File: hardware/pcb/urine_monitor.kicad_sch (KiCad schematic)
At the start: 27 parts, among them J1 LoadCell, J2 EInk_FPC, J3 USB-C_Power, J4 I2C+BOOT0+PWR, Q1 SI2301, Q2 2N7002, SW1 USER_BTN, U1 RAK3172, U2 HX711, U3 TPS61220, U4 MIC5504-3.3

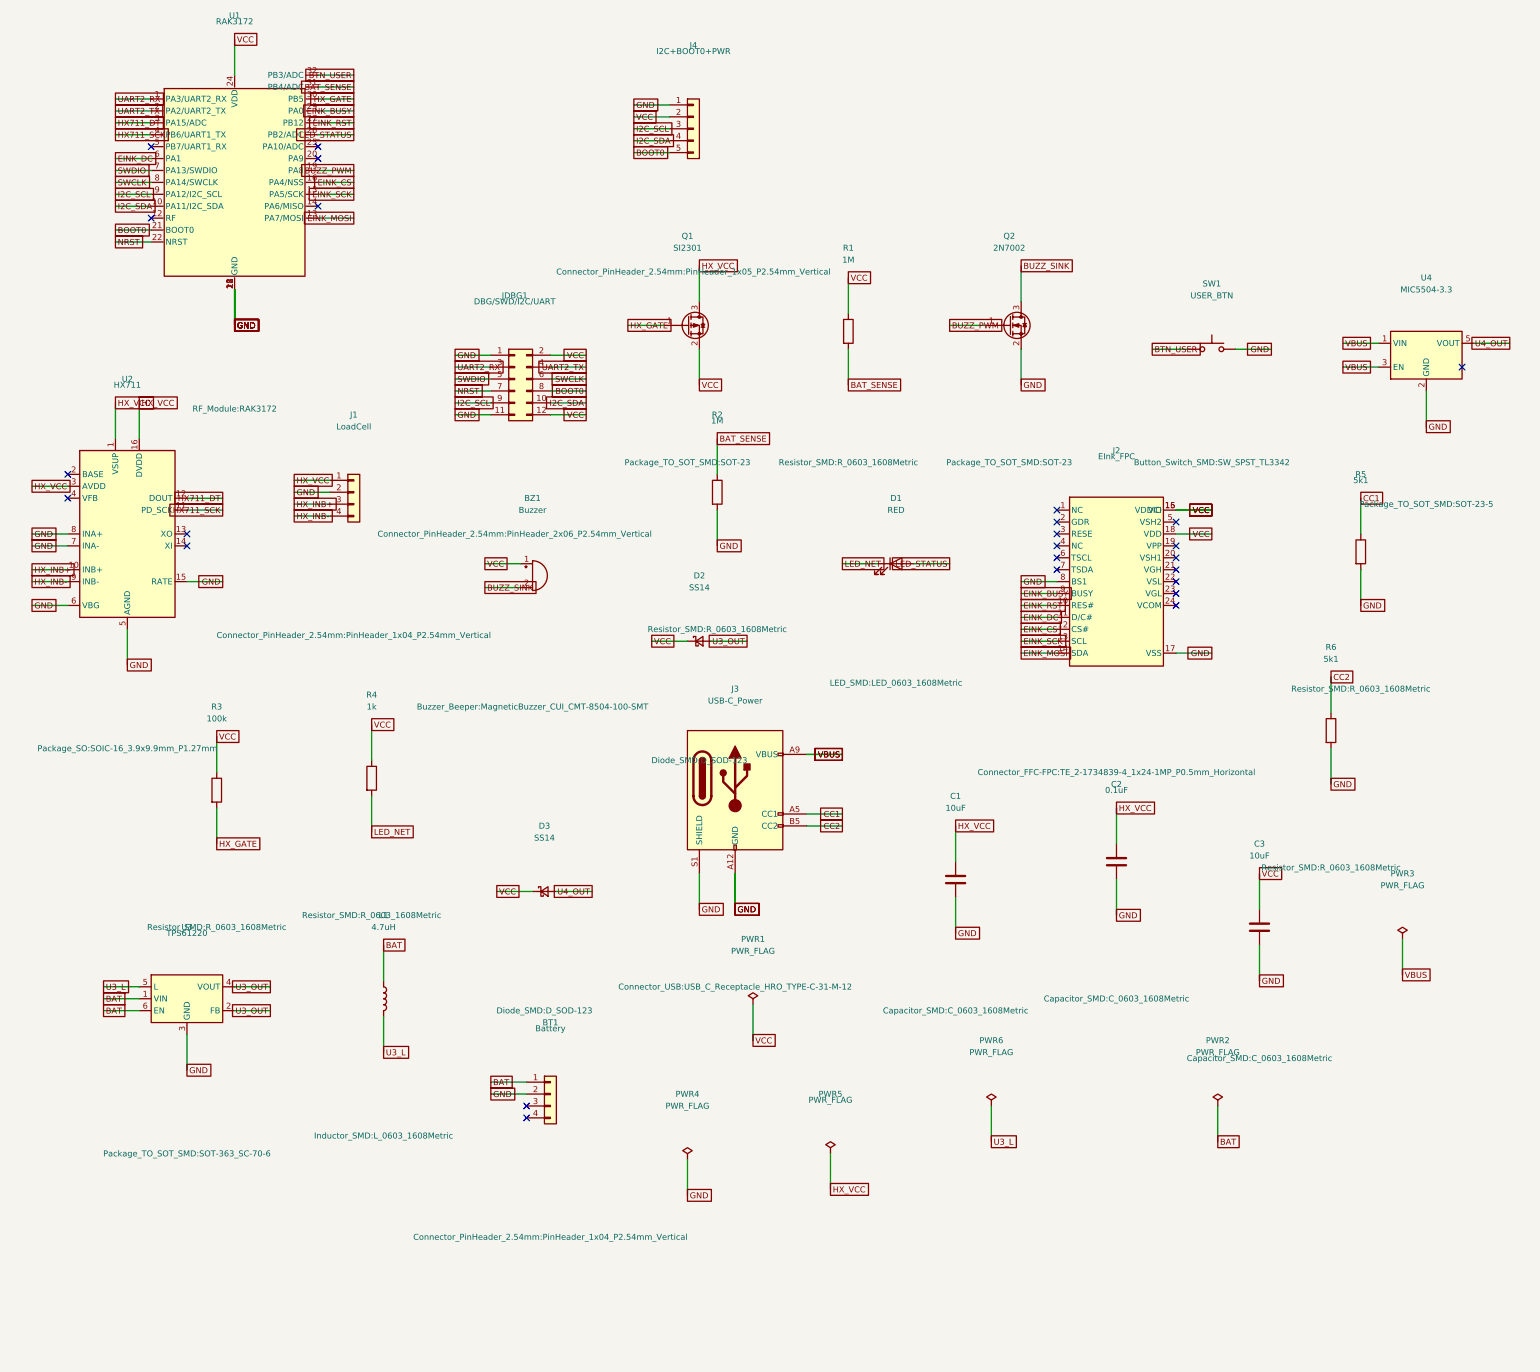
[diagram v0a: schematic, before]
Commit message: init
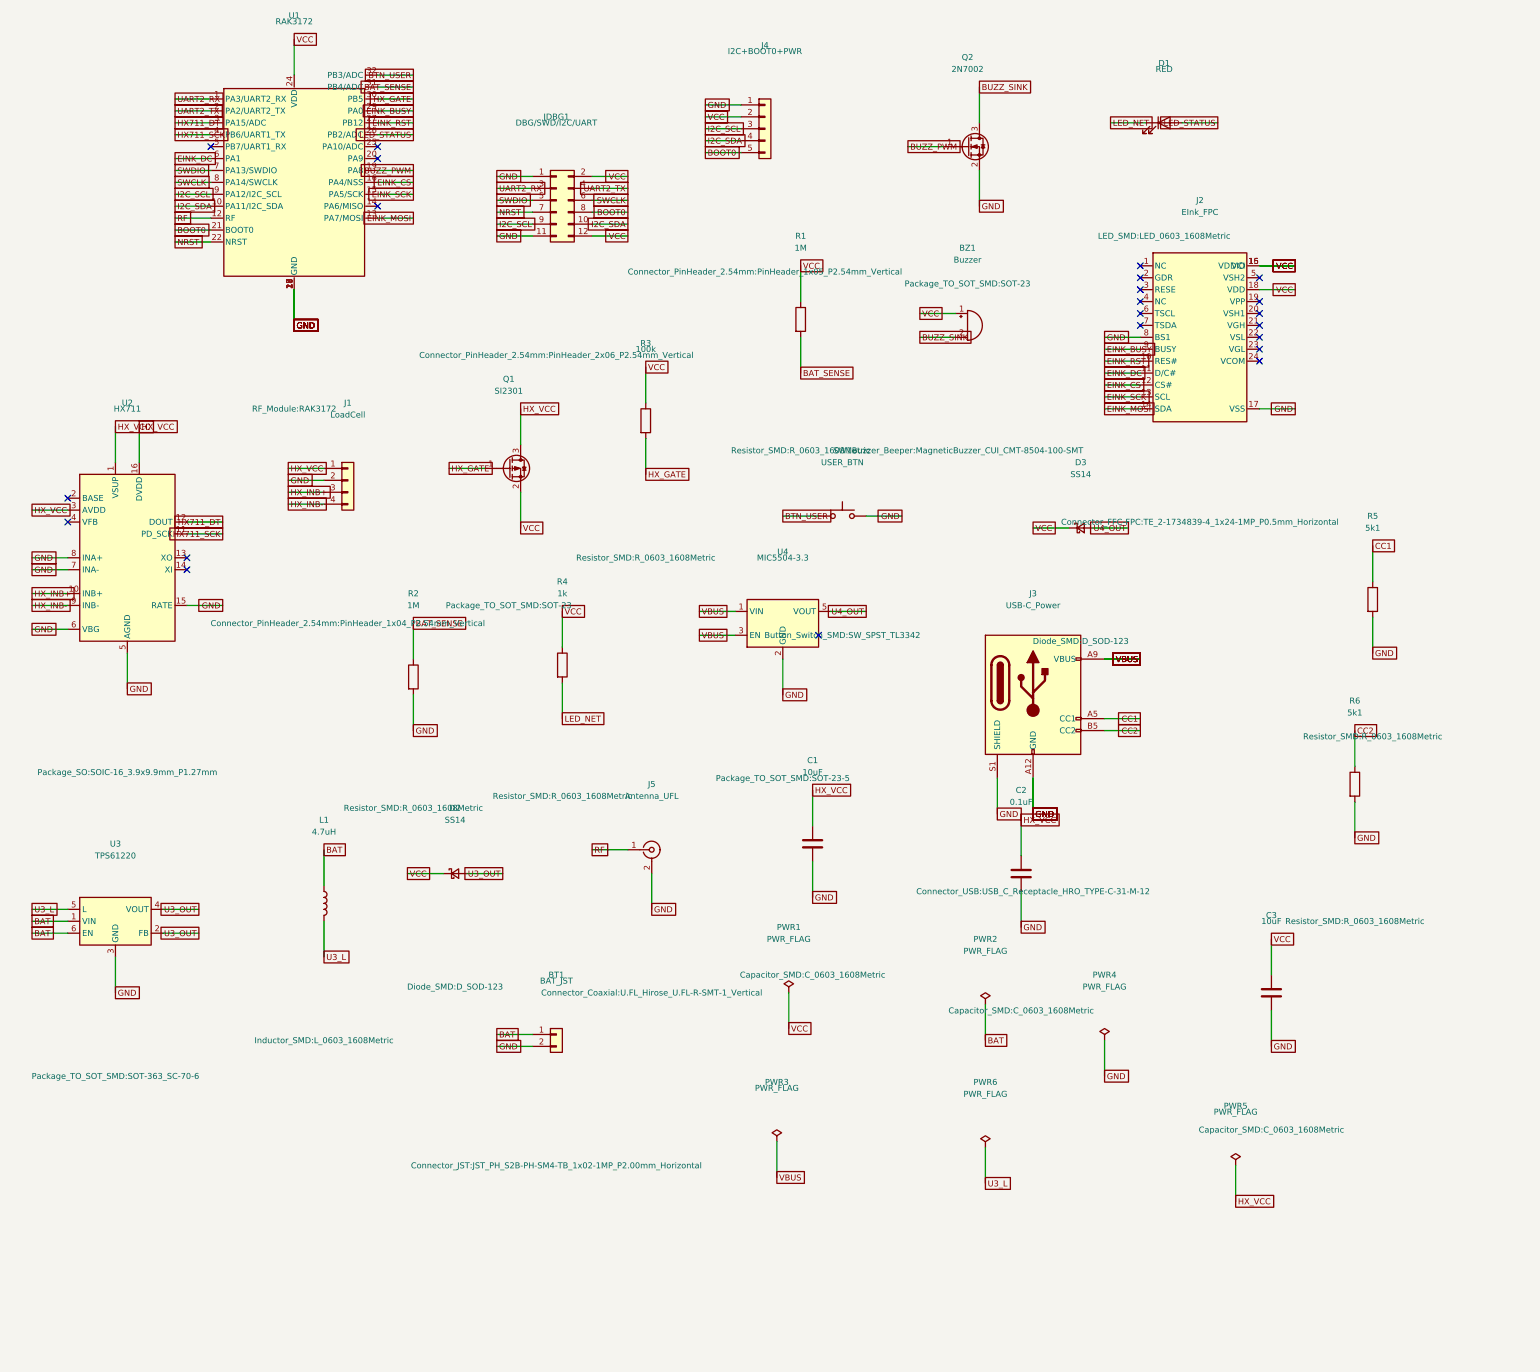
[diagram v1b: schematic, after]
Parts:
- removed BT1: Battery, Connector_PinHeader_2.54mm:PinHeader_1x04_P2.54mm_Vertical, symbol Connector_Generic:Conn_01x04
- removed J3: USB-C_Power, Connector_USB:USB_C_Receptacle_HRO_TYPE-C-31-M-12, symbol Connector:USB_C_Receptacle_PowerOnly_6P
- added BT1: BAT_JST, Connector_JST:JST_PH_S2B-PH-SM4-TB_1x02-1MP_P2.00mm_Horizontal, symbol Connector_Generic:Conn_01x02
- added J3: USB-C_Power, Connector_USB:USB_C_Receptacle_HRO_TYPE-C-31-M-12, symbol Connector:USB_C_Receptacle_PowerOnly_24P
- added J5: Antenna_UFL, Connector_Coaxial:U.FL_Hirose_U.FL-R-SMT-1_Vertical, symbol Connector:Conn_Coaxial
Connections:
- net BAT: now also BT1.1 (Pin_1)
- net CC1: now also J3.A5 (CC1)
- net CC2: now also J3.B5 (CC2)
- net GND: now also BT1.2 (Pin_2), J3.A1 (GND), J3.A12 (GND), J3.B1 (GND), J3.B12 (GND), J3.S1 (SHIELD), J5.2 (Ext)
- net VBUS: now also J3.A4 (VBUS), J3.A9 (VBUS), J3.B4 (VBUS), J3.B9 (VBUS)
- net RF: now reaches U1.12 (RF)
- net RF: now also J5.1 (In)
- no-connect marks 25 -> 22

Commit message: init
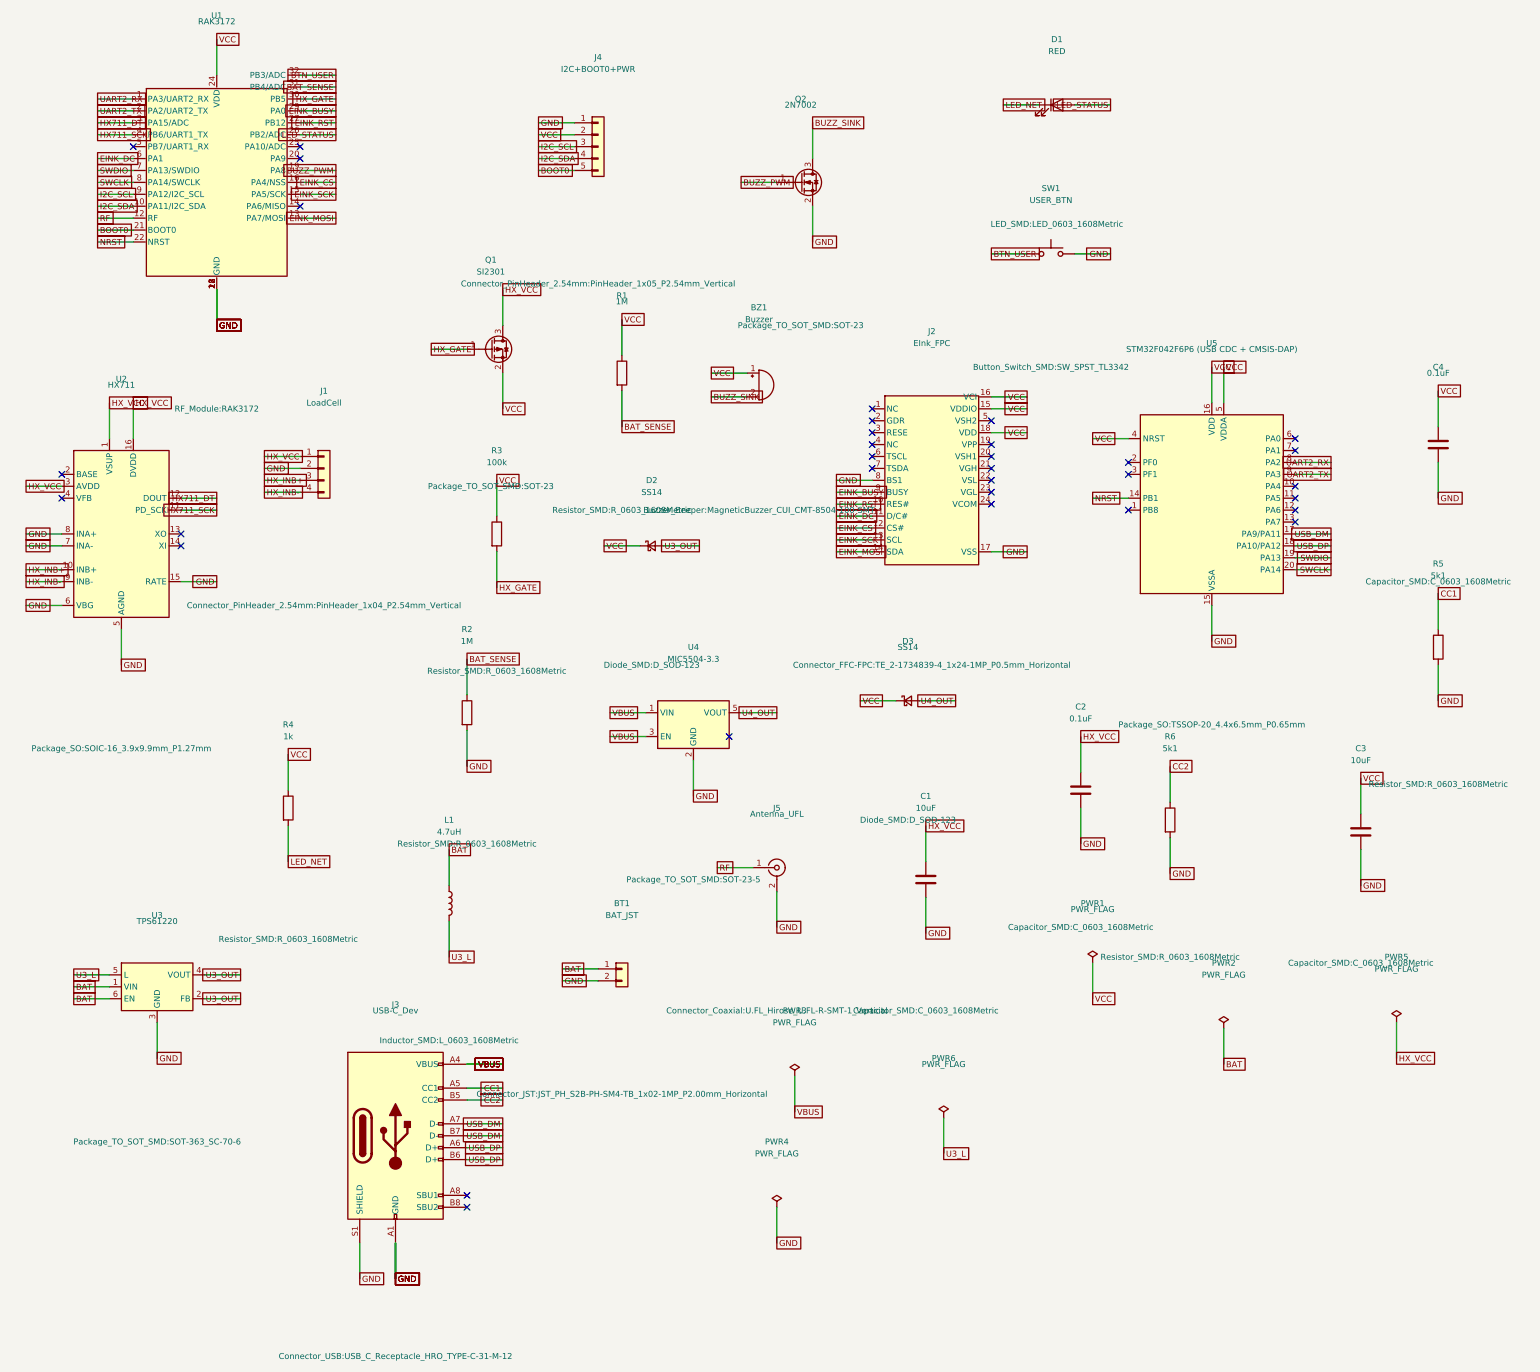
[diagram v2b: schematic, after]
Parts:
- removed J3: USB-C_Power, Connector_USB:USB_C_Receptacle_HRO_TYPE-C-31-M-12, symbol Connector:USB_C_Receptacle_PowerOnly_24P
- removed JDBG1: DBG/SWD/I2C/UART, Connector_PinHeader_2.54mm:PinHeader_2x06_P2.54mm_Vertical, symbol Connector_Generic:Conn_02x06_Odd_Even
- added C4: 0.1uF, Capacitor_SMD:C_0603_1608Metric, symbol Device:C
- added J3: USB-C_Dev, Connector_USB:USB_C_Receptacle_HRO_TYPE-C-31-M-12, symbol Connector:USB_C_Receptacle_USB2.0_16P
- added U5: STM32F042F6P6 (USB CDC + CMSIS-DAP), Package_SO:TSSOP-20_4.4x6.5mm_P0.65mm, symbol MCU_ST_STM32F0:STM32F042F6Px
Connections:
- net CC1: now also J3.A5 (CC1)
- net CC2: now also J3.B5 (CC2)
- net GND: now also C4.2, J3.A1 (GND), J3.A12 (GND), J3.B1 (GND), J3.B12 (GND), J3.S1 (SHIELD), U5.15 (VSSA)
- net NRST: now also U5.14 (PB1)
- net SWCLK: now also U5.20 (PA14)
- net SWDIO: now also U5.19 (PA13)
- net UART2_RX: now also U5.8 (PA2)
- net UART2_TX: now also U5.9 (PA3)
- net VBUS: now also J3.A4 (VBUS), J3.A9 (VBUS), J3.B4 (VBUS), J3.B9 (VBUS)
- net VCC: now also C4.1, U5.16 (VDD), U5.4 (NRST), U5.5 (VDDA)
- new net USB_DM: J3.A7 (D-), J3.B7 (D-), U5.17 (PA9/PA11)
- new net USB_DP: J3.A6 (D+), J3.B6 (D+), U5.18 (PA10/PA12)
- no-connect marks 22 -> 33
